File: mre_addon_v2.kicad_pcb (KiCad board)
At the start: 2 copper layers, 80.6 x 48.4 mm, 86 parts, among them J1 TC2030, J10 Molex_Micro-Fit_3.0_43045-080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, J10 Molex_Micro-Fit_3.0_43045-081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, J15 microSD_HC_Wuerth_693072010801, J15x MICRO-SDCARD-CONNECTOR-330006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, J2 Conn_01x06_Male, J20 Conn_02x05_Odd_Even-Connector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, J21 Soldering PAD for 12V_MREL, J3 Conn_01x03_Male, J30 Conn_02x05_Odd_Even-Connector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, J40 CONN_Molex, J40x Molex_Micro-Fit_3.0_43045-021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, J41 CONN_Sparkfun, Q1 BTS3028, SW1 SW_Push, U0 wideband_MRE_R055, U1 STM32F072CBUx, U2 MCP6004, U3 AD8628, U3 SO-8_3.9x4.9mm_P1.27mm, U4 REF3033, U5 TJA1051T-3, U6 MAX31855KASA

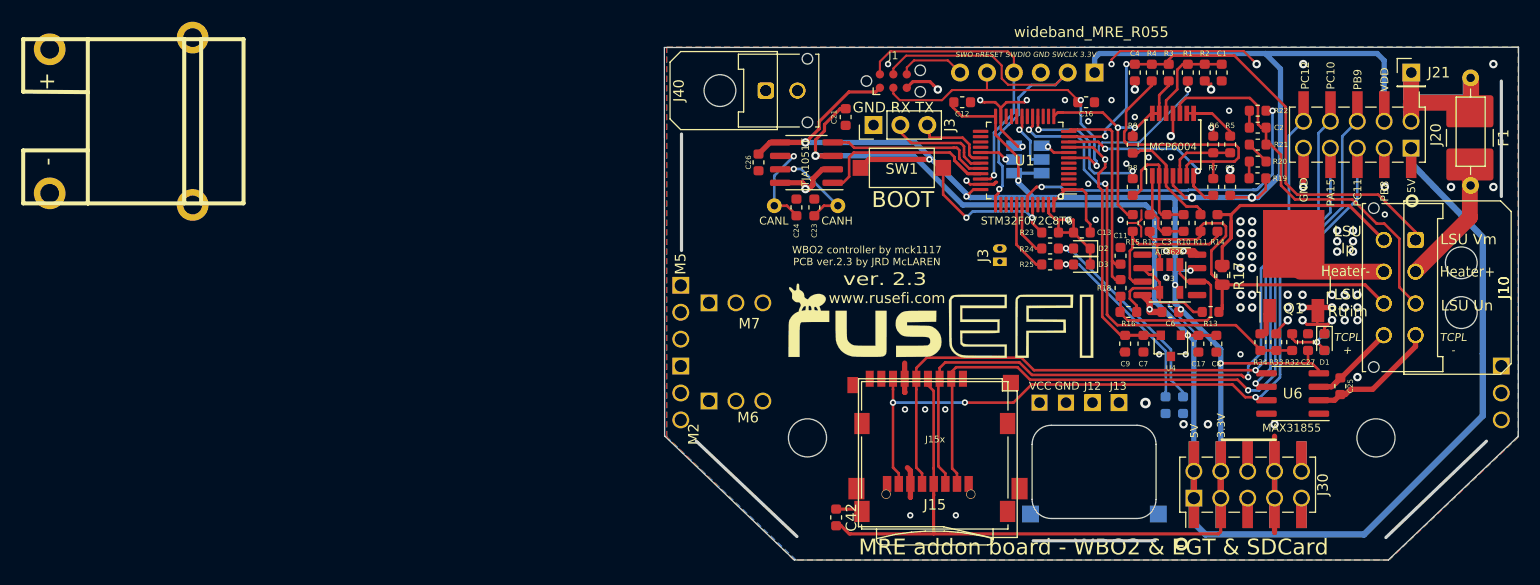
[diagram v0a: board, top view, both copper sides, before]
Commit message: Add files via upload
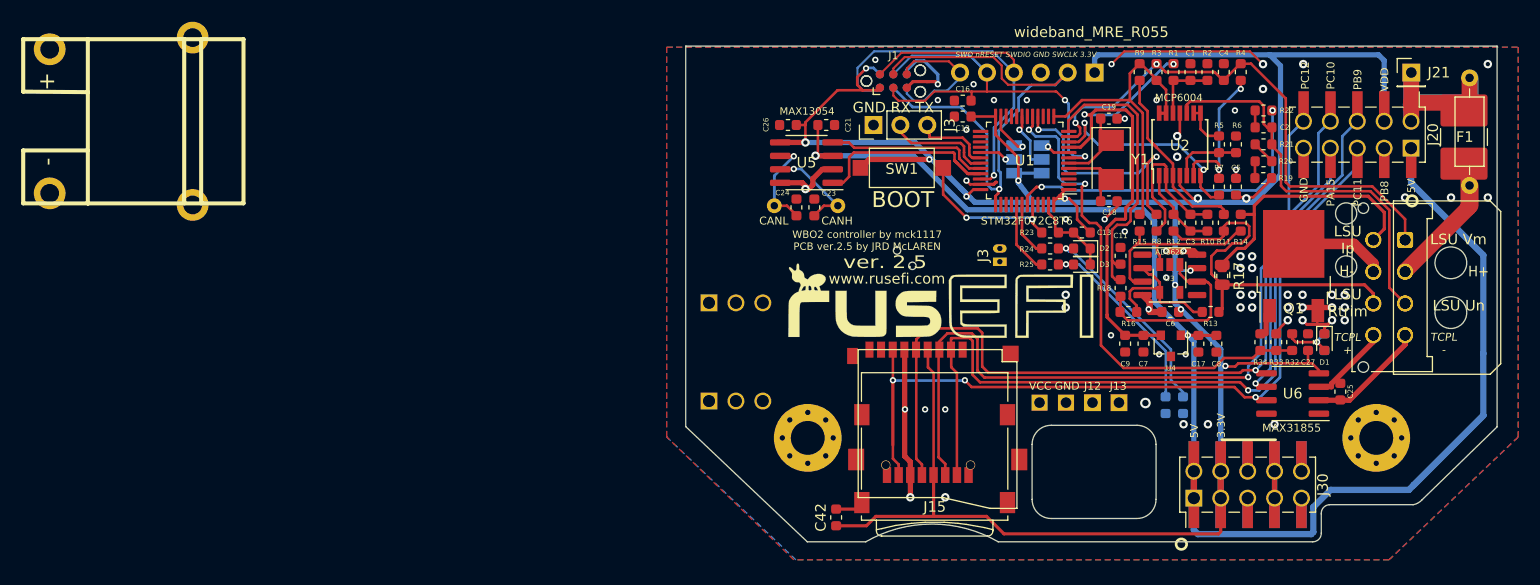
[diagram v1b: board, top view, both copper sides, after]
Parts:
- removed J40: CONN_Molex, Connector_Molex:Molex_Micro-Fit_3.0_43045-0200_2x01_P3.00mm_Horizontal
- removed J40x: Molex_Micro-Fit_3.0_43045-0212_2x01_P3.00mm_Vertical, Connector_Molex:Molex_Micro-Fit_3.0_43045-0212_2x01_P3.00mm_Vertical
- added ?: , , F.Cu at (90.0, 147.3)
- added ?: , , F.Cu at (88.8, 146.2)
- added C18: 18pF, Capacitor_SMD:C_0603_1608Metric, F.Cu at (117.0, 140.3)
- added C19: 18pF, Capacitor_SMD:C_0603_1608Metric, F.Cu at (117.0, 132.6)
- added H1: MountingHole_3.2mm_M3_Pad_Via, MountingHole:MountingHole_3.2mm_M3_Pad_Via, F.Cu at (88.5, 162.7)
- added H2: MountingHole_3.2mm_M3_Pad_Via, MountingHole:MountingHole_3.2mm_M3_Pad_Via, F.Cu at (142.2, 162.7)
- added J1: TC2030, rusefi_lib:Tag-Connect_TC2030-IDC-NL_2x03_P1.27mm_Vertical, B.Cu at (96.6, 129.0)
- added Y1: 8MHz, Crystal:Crystal_SMD_5032-2Pin_5.0x3.2mm, F.Cu at (117.2, 136.4)
- J10: value Molex_Micro-Fit_3.0_43045-0812_2x04_P3.00mm_Vertical -> Molex_Micro-Fit_3.0_43045-0800_43045-0812
- moved LOGO1 49.0 mm to (91.4, 169.1)
- moved C16 11.7 mm to (103.2, 130.8), turned to 180 degrees
- moved R4 8.40 mm to (129.4, 128.2)
- moved C4 8.40 mm to (127.8, 128.2), turned to 90 degrees
- moved R9 6.89 mm to (119.8, 128.2)
- moved C26 4.49 mm to (86.7, 133.2), turned to 180 degrees
- moved R8 4.06 mm to (121.5, 142.4)
- moved C1 2.95 mm to (124.7, 128.2), turned to 90 degrees
- moved J15x 2.75 mm to (100.8, 161.8)
- moved R12 2.25 mm to (123.0, 142.4)
- moved C3 2.25 mm to (124.7, 142.4)
- moved R10 2.25 mm to (126.2, 142.4)
- moved R11 2.20 mm to (127.8, 142.4)
- moved R14 2.20 mm to (129.4, 142.4)
- moved R6 2.15 mm to (128.9, 135.0)
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- renumbered U3 to U3x
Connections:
- J15 pad 1: Net-(J15-Pad1) -> unconnected-(J15-Pad1)
- J15 pad 8: Net-(J15-Pad8) -> unconnected-(J15-Pad8)
- U1 pad 14: Net-(U1-Pad14) -> unconnected-(U1-Pad14)
- U1 pad 15: Net-(U1-Pad15) -> unconnected-(U1-Pad15)
- U1 pad 18: Net-(U1-Pad18) -> unconnected-(U1-Pad18)
- U1 pad 2: Net-(U1-Pad2) -> unconnected-(U1-Pad2)
- U1 pad 20: Net-(U1-Pad20) -> unconnected-(U1-Pad20)
- U1 pad 21: Net-(U1-Pad21) -> unconnected-(U1-Pad21)
- U1 pad 22: Net-(U1-Pad22) -> unconnected-(U1-Pad22)
- U1 pad 25: Net-(U1-Pad25) -> unconnected-(U1-Pad25)
- U1 pad 26: Net-(U1-Pad26) -> unconnected-(U1-Pad26)
- U1 pad 27: Net-(U1-Pad27) -> unconnected-(U1-Pad27)
- U1 pad 28: Net-(U1-Pad28) -> unconnected-(U1-Pad28)
- U1 pad 3: Net-(U1-Pad3) -> unconnected-(U1-Pad3)
- U1 pad 38: Net-(U1-Pad38) -> unconnected-(U1-Pad38)
- U1 pad 39: Net-(U1-Pad39) -> unconnected-(U1-Pad39)
- U1 pad 4: Net-(U1-Pad4) -> unconnected-(U1-Pad4)
- U1 pad 40: Net-(U1-Pad40) -> unconnected-(U1-Pad40)
- U1 pad 45: Net-(U1-Pad45) -> unconnected-(U1-Pad45)
- U1 pad 46: Net-(U1-Pad46) -> unconnected-(U1-Pad46)
- U6 pad 8: Net-(U6-Pad8) -> unconnected-(U6-Pad8)
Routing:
- net /mcu_adc_mre_wbo2_v2/SWDIO: track 27.8 -> 47.1 mm
- net /mcu_adc_mre_wbo2_v2/SWCLK: track 36.9 -> 53.3 mm
- net Net-(R4-Pad2): track 27.2 -> 14.6 mm, vias 0 -> 2
- net GND: track 105.1 -> 94.5 mm, vias 85 -> 65
- net /mcu_adc_mre_wbo2_v2/nRESET: track 30.7 -> 41.0 mm
- net /mcu_adc_mre_wbo2_v2/Ip_dac: track 14.2 -> 22.7 mm
- net VDDA: track 38.7 -> 46.0 mm
- net Net-(C19-Pad2): track 0.00 -> 6.95 mm
- net Net-(C18-Pad2): track 0.00 -> 6.90 mm
- net /mcu_adc_mre_wbo2_v2/Ip_sense: track 20.3 -> 27.2 mm
- net Net-(R11-Pad2): track 11.5 -> 18.3 mm
- net /mcu_adc_mre_wbo2_v2/SWO: track 6.42 -> 13.1 mm
- net +5V: track 141.5 -> 147.8 mm
- net /can_fet_egt_sd_v2/PC11: track 74.5 -> 80.5 mm
- net /can_fet_egt_sd_v2/PB9: track 70.2 -> 75.7 mm
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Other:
- board size 80.6 x 48.4 mm -> 76.6 x 46.8 mm
- net class Default removed
- board text added: "H+"
- board text added: "H-"
- board text added: "MAX13054"
- board text added: "WBO2 controller by mck1117 PCB ver.2.5 by JRD McLAREN"
- board text added: "ver. 2.5"
- board text removed: "Heater+"
- board text removed: "Heater-"
- board text removed: "TJA1051T"
- board text removed: "WBO2 controller by mck1117 PCB ver.2.3 by JRD McLAREN"
- board text removed: "ver. 2.3"
